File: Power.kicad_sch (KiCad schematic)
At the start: 11 parts, among them IC5 LM74502HDDFR, Q5 PSMN8R5-40MSDX

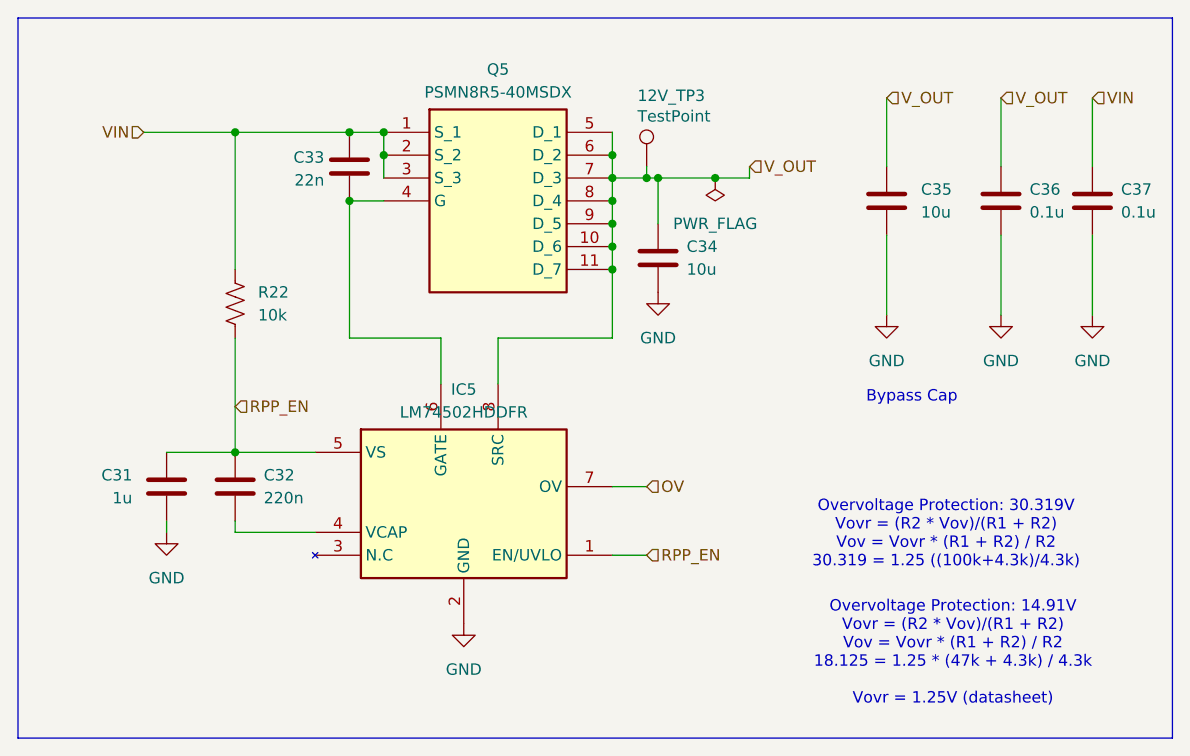
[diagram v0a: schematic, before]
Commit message: RevA8 layout changes
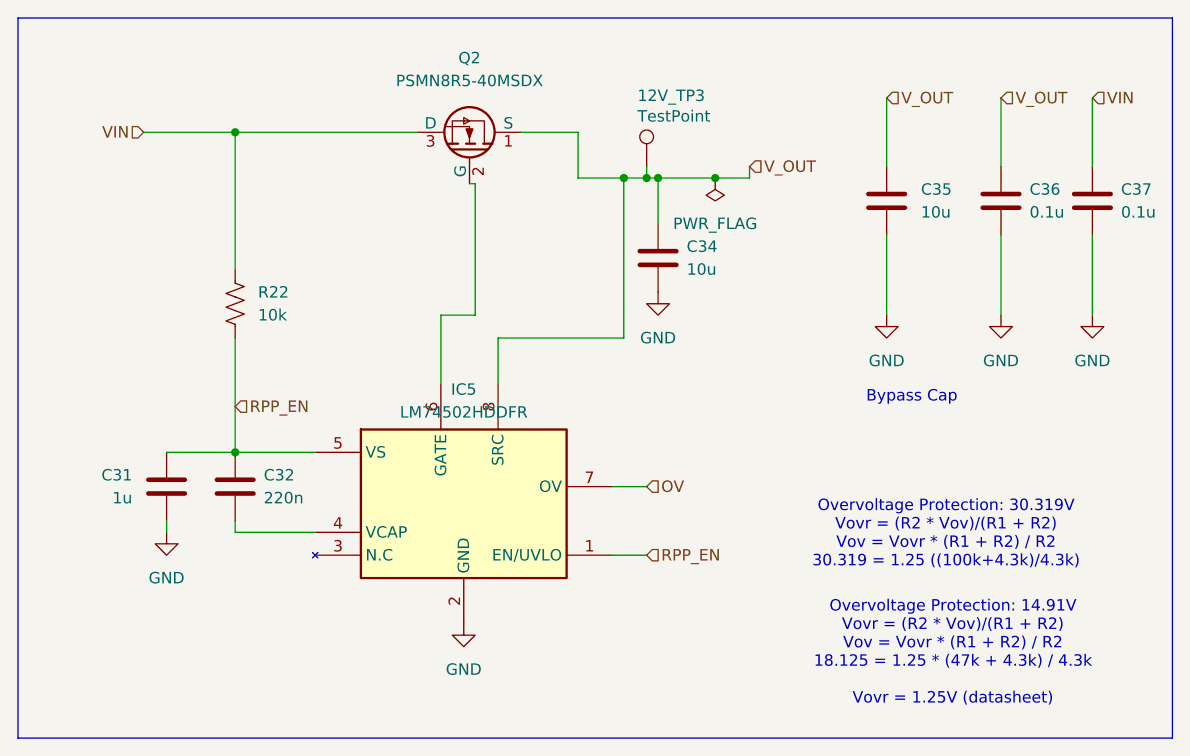
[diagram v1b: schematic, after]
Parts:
- removed C33: 22n, Capacitor_SMD:C_0603_1608Metric, symbol Device:C
- removed Q5: PSMN8R5-40MSDX, UTSVT_Power:PSMN8R5-40MSDX, symbol UTSVT_Power:PSMN8R5-40MSDX
- added Q2: PSMN8R5-40MSDX, UTSVT_Power:PSMN8R5-40MSDX, symbol utsvt_power:PSMN8R5-40MSDX
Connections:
- net VIN: now also Q2.3 (D)
- net V_OUT: now also Q2.1 (S)
- net at IC5.6 (GATE): now also Q2.2 (G)
